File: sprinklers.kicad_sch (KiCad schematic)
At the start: 37 parts, among them J2 Conn_Coaxial_Power, K1 SANYOU_SRD_Form_C, K2 SANYOU_SRD_Form_C, K3 SANYOU_SRD_Form_C, K4 SANYOU_SRD_Form_C, K5 SANYOU_SRD_Form_C, K6 SANYOU_SRD_Form_C, Q1 Q_NMOS_GDS, Q2 Q_NMOS_GDS, Q3 Q_NMOS_GDS, Q4 Q_NMOS_GDS, Q5 Q_NMOS_GDS, Q6 Q_NMOS_GDS, U1 LM2596S-5, U2 ESP32-WROOM-32D, U3 AP1117-33

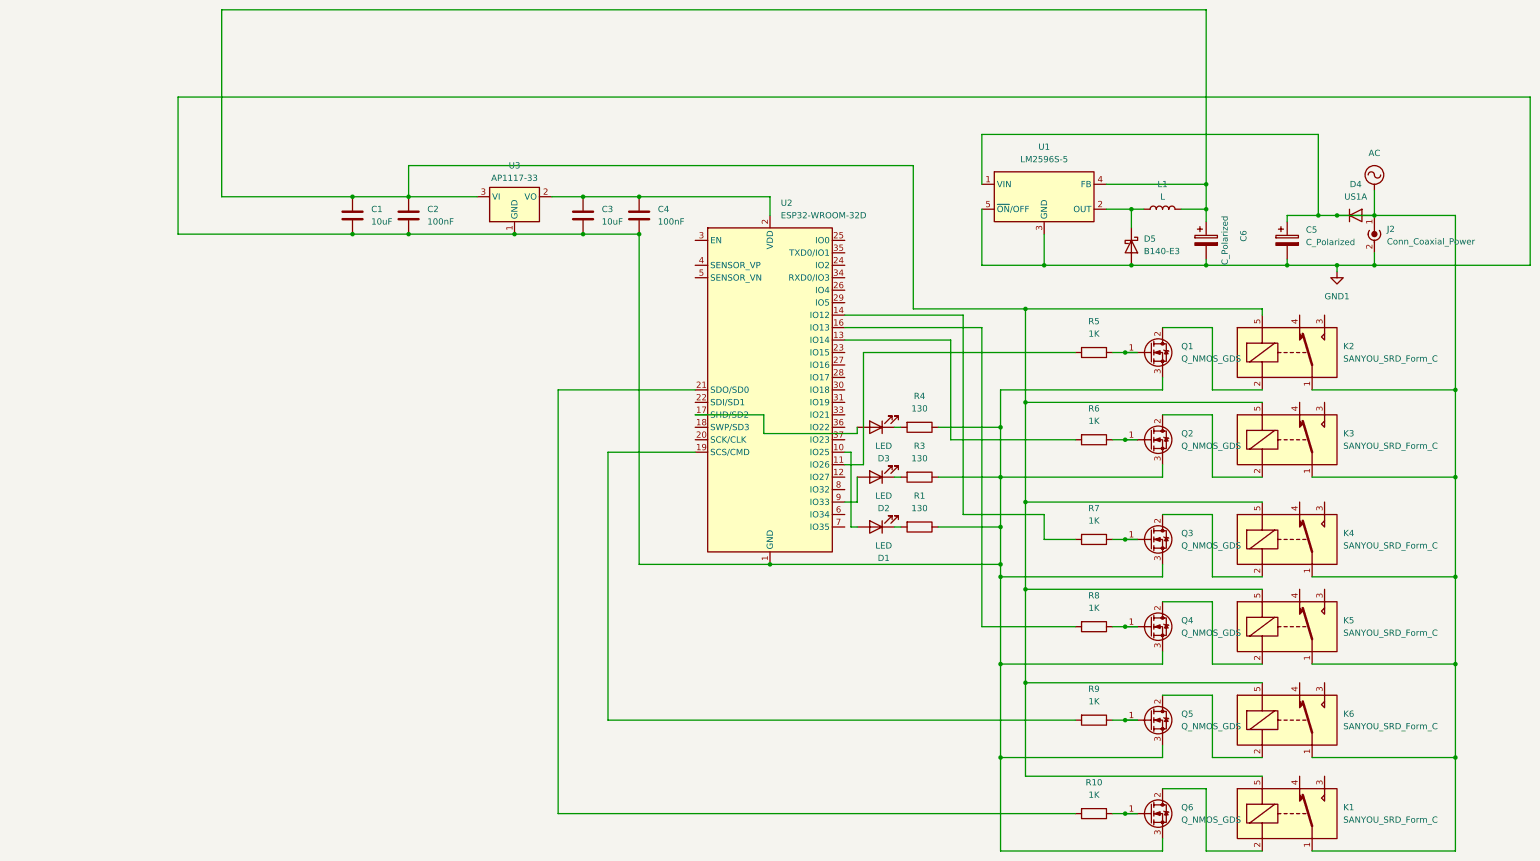
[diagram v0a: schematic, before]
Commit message: orgenize schematic
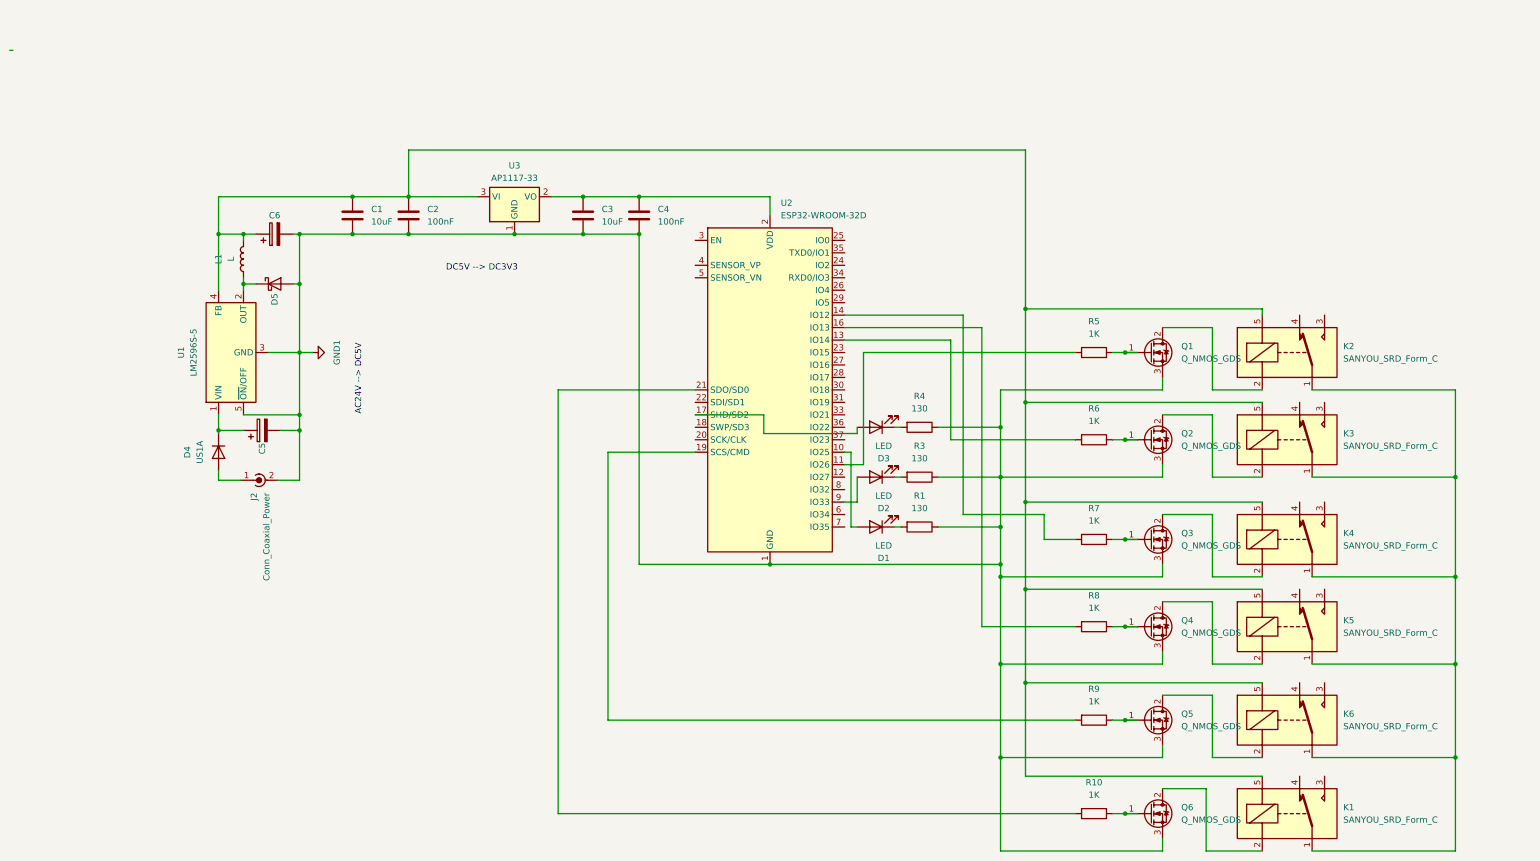
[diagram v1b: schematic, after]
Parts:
- D1: LCSC C2297 -> C84256
- D3: LCSC C84256 -> C2297
- D5: LCSC (none) -> C968568
- R4: LCSC C4410 -> C17451
- R8: LCSC C17451 -> C4410
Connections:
- net AC: no longer names the net of K1.1, K2.1, K3.1, K4.1, K5.1, K6.1
- net AC: no longer C5.1, D4.1 (K), D4.2 (A), J2.1 (In), U1.1 (VIN)
- new net: C5.1, D4.1 (K), U1.1 (VIN)
- new net: D4.2 (A), J2.1 (In)
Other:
- note added: "AC24V --> DC5V"
- note added: "DC5V --> DC3V3"
- moved on the sheet: C5, C6, D4, D5, J2, L1, U1
